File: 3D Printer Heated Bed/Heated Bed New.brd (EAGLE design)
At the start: 74.6 x 55.9 mm, 18 parts, among them IC1 7805T, IC2 ATMEGA168-20P, Q1 16Mhz, Q2 IRF530, X1 1751248, X2 1751248, X3 1751248

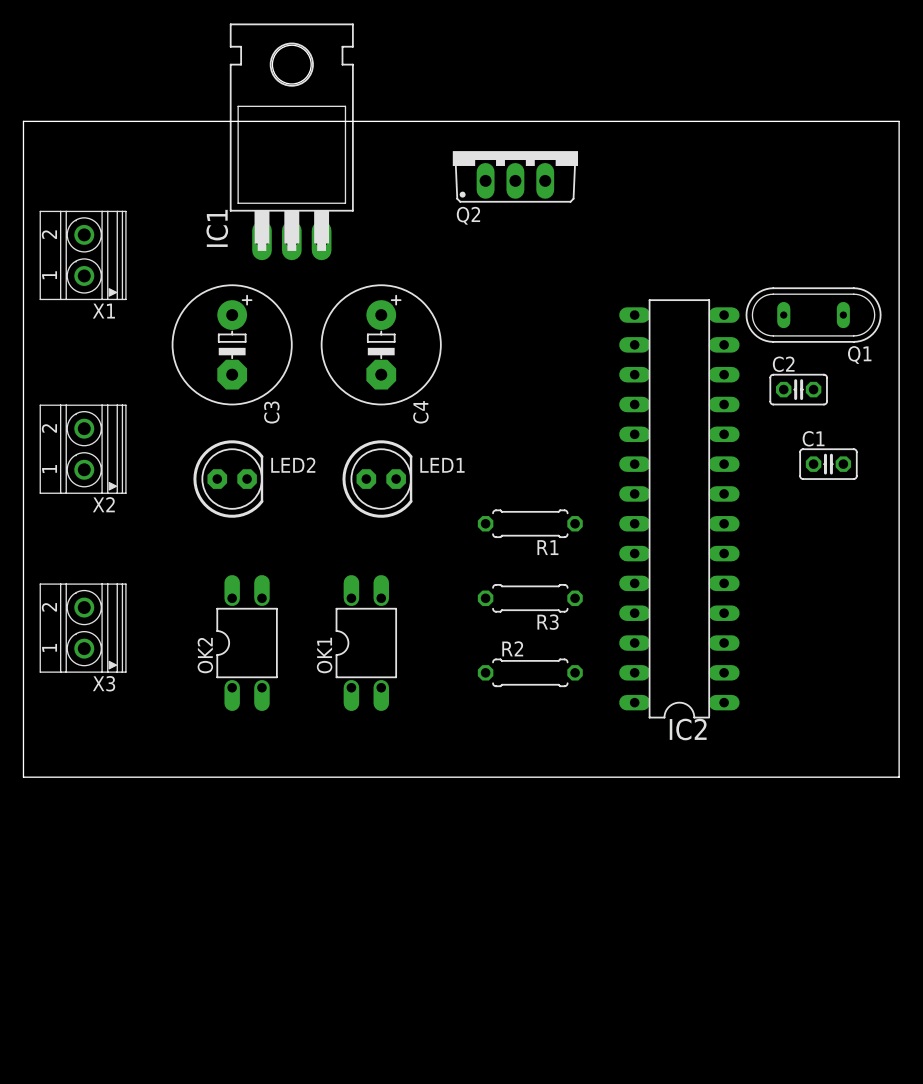
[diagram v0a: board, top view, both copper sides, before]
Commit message: Update
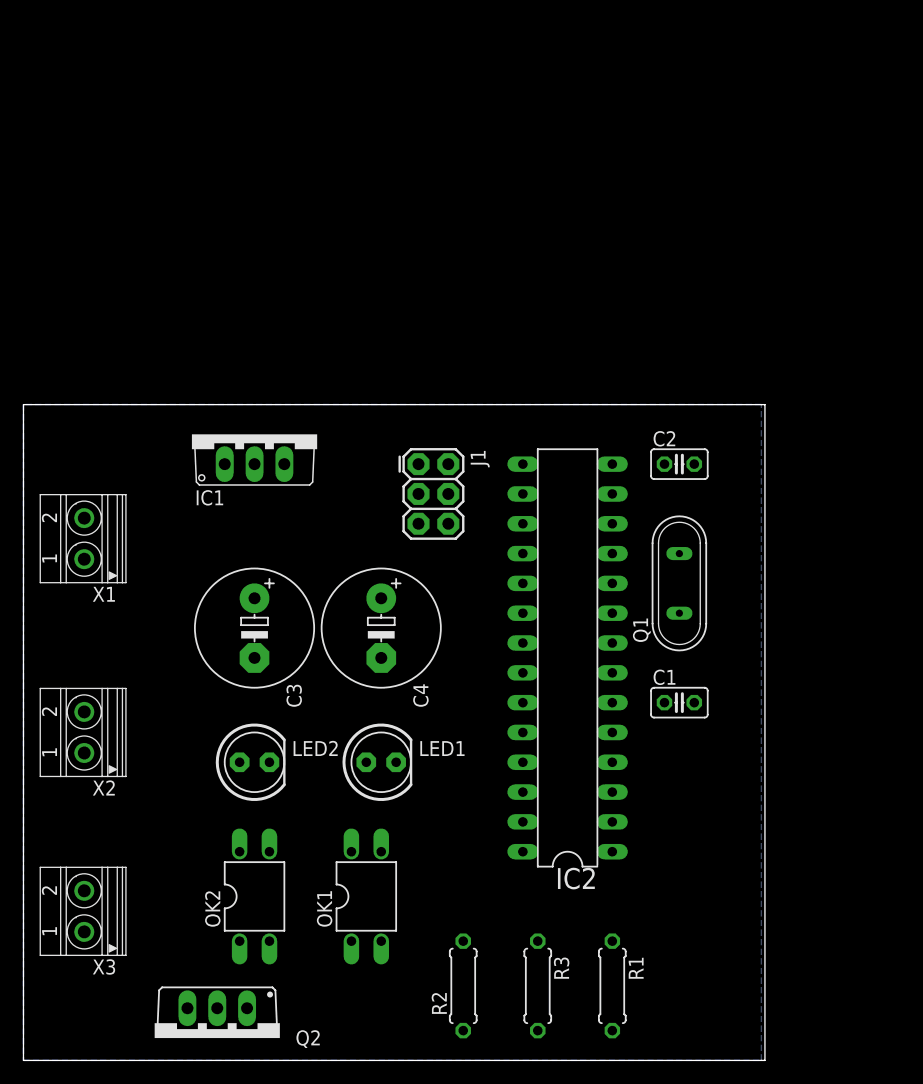
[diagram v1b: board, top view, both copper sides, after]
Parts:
- added J1: AVR_SPI_PRG_6PTH, SparkFun-Connectors:2X3
- IC1: value 7805T -> 7805TV; device linear:TO220H -> linear:TO220V
- moved Q2 79.7 mm to (16.5, 1.91), turned to 180 degrees
- moved R1 40.0 mm to (50.2, 6.35), turned to 270 degrees
- moved R3 33.0 mm to (43.8, 6.35), turned to 270 degrees
- moved R2 27.3 mm to (37.5, 6.35), turned to 90 degrees
- moved IC1 26.9 mm to (19.7, 53.3)
- moved Q1 25.6 mm to (55.9, 40.6), turned to 90 degrees
- moved C3 24.2 mm to (19.7, 36.8)
- moved LED2 24.2 mm to (19.7, 25.4)
- moved C4 24.1 mm to (30.5, 36.8)
- moved LED1 24.1 mm to (30.5, 25.4)
- moved X2 24.1 mm to (5.08, 27.9)
- moved X3 24.1 mm to (5.08, 12.7)
- moved X1 24.1 mm to (5.08, 44.5)
- moved C1 24.0 mm to (55.9, 30.5)
- moved OK2 21.6 mm to (19.7, 14.0)
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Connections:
- new net MISO: IC2.18, J1.1
- new net MOSI: IC2.17, J1.4
- new net RESET: IC2.1, J1.5
- new net SCK: IC2.19, J1.3
- net 5V: now also J1.2
- net GND: now also J1.6
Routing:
- added copper zone on layer 16, net GND
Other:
- board size 74.6 x 55.9 mm -> 63.2 x 55.9 mm
